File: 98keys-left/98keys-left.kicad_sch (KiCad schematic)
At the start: 115 parts, among them J1 Conn_01x04_Male, SW1 MX-NO-LED, SW10 MX-NO-LED, SW11 MX-NO-LED, SW12 MX-NO-LED, SW13 MX-NO-LED, SW14 MX-NO-LED, SW15 MX-NO-LED, SW16 MX-NO-LED, SW17 MX-NO-LED, SW18 MX-NO-LED, SW19 MX-NO-LED, SW2 MX-NO-LED, SW20 MX-NO-LED, SW21 MX-NO-LED, SW22 MX-NO-LED, SW23 MX-NO-LED, SW24 MX-NO-LED, SW25 MX-NO-LED, SW26 MX-NO-LED, SW27 MX-NO-LED, SW28 MX-NO-LED, SW29 MX-NO-LED, SW3 MX-NO-LED, SW30 MX-NO-LED, SW31 MX-NO-LED, SW32 MX-NO-LED, SW33 MX-NO-LED, SW34 MX-NO-LED, SW35 MX-NO-LED, SW36 MX-NO-LED, SW37 MX-NO-LED, SW38 MX-NO-LED, SW39 MX-NO-LED, SW4 MX-NO-LED, SW40 MX-NO-LED, SW41 MX-NO-LED, SW42 MX-NO-LED, SW43 MX-NO-LED, SW44 MX-NO-LED, SW45 MX-NO-LED, SW46 MX-NO-LED, SW47 MX-NO-LED, SW48 SW_Push, SW5 MX-NO-LED, SW6 MX-NO-LED, SW7 MX-NO-LED, SW8 MX-NO-LED, SW9 MX-NO-LED, U1 Pico

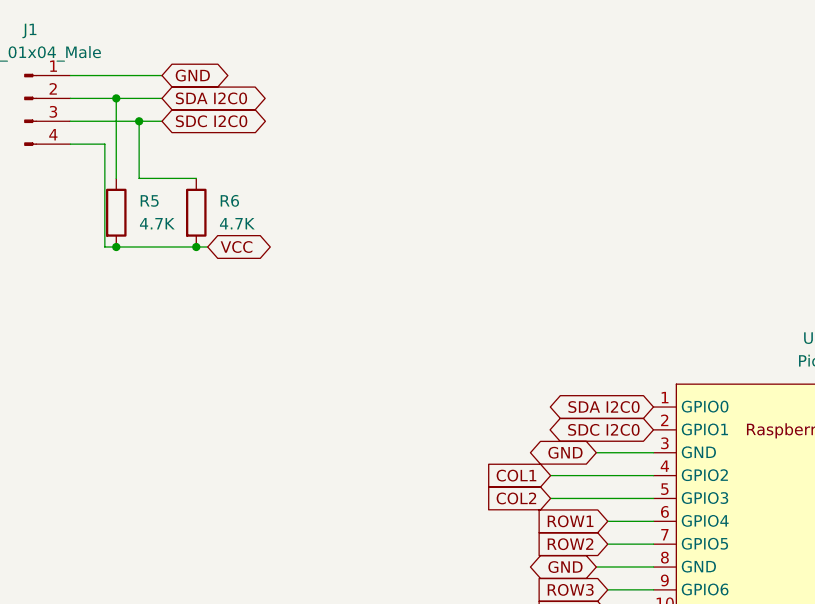
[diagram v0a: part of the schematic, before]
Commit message: Add files via upload
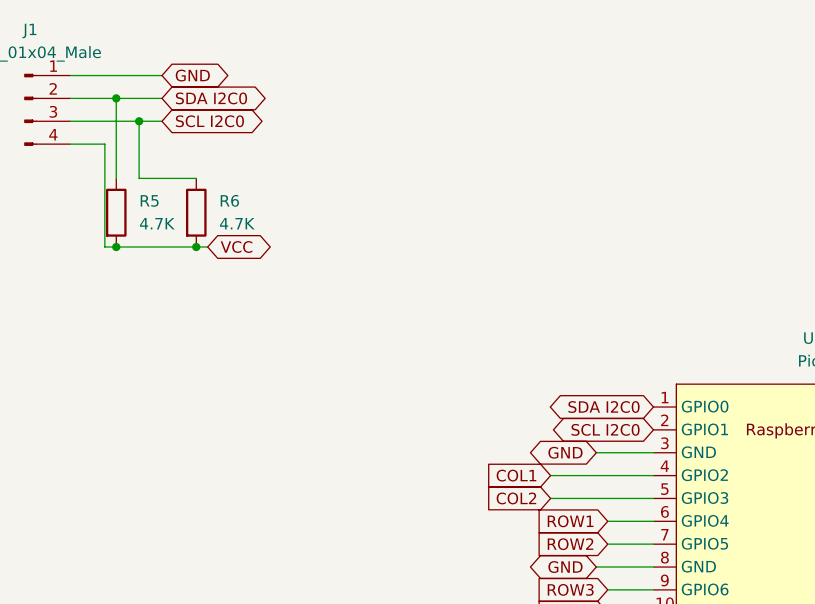
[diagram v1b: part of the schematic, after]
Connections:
- net SDC I2C0 renamed SCL I2C0
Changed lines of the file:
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@@
     )
   )
-  (global_label "SDC I2C0" (shape bidirectional) (at 495.3 86.36 180) (fields_autoplaced)
+  (global_label "SCL I2C0" (shape bidirectional) (at 495.3 86.36 180) (fields_autoplaced)
     (effects (font (size 1.27 1.27)) (justify right))
-    (property "Intersheet References" "${INTERSHEET_REFS}" (id 0) (at 483.9648 86.4394 0)
+    (property "Intersheet References" "${INTERSHEET_REFS}" (id 0) (at 484.2068 86.2806 0)
       (effects (font (size 1.27 1.27)) (justify right) hide)
     )
@@
     )
   )
-  (global_label "SDC I2C0" (shape bidirectional) (at 440.69 52.07 0) (fields_autoplaced)
+  (global_label "SCL I2C0" (shape bidirectional) (at 440.69 52.07 0) (fields_autoplaced)
     (effects (font (size 1.27 1.27)) (justify left))
-    (property "Intersheet References" "${INTERSHEET_REFS}" (id 0) (at 452.0252 51.9906 0)
+    (property "Intersheet References" "${INTERSHEET_REFS}" (id 0) (at 451.7832 51.9906 0)
       (effects (font (size 1.27 1.27)) (justify left) hide)
     )

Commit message: Add files via upload
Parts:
- J1: footprint Connector_PinHeader_2.54mm:PinHeader_1x04_P2.54mm_Vertical -> Connector_Audio:Jack_3.5mm_CUI_SJ1-43514_Horizontal
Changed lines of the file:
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@@
     (property "Reference" "J1" (id 0) (at 426.085 41.91 0))
     (property "Value" "Conn_01x04_Male" (id 1) (at 426.085 44.45 0))
-    (property "Footprint" "Connector_PinHeader_2.54mm:PinHeader_1x04_P2.54mm_Vertical" (id 2) (at 425.45 49.53 0)
+    (property "Footprint" "Connector_Audio:Jack_3.5mm_CUI_SJ1-43514_Horizontal" (id 2) (at 425.45 49.53 0)
       (effects (font (size 1.27 1.27)) hide)
     )
@@
     )
     (path "/b1a2f4f8-5ce5-4e86-9c1b-c2a387c5d74f"
-      (reference "J1") (unit 1) (value "Conn_01x04_Male") (footprint "Connector_PinHeader_2.54mm:PinHeader_1x04_P2.54mm_Vertical")
+      (reference "J1") (unit 1) (value "Conn_01x04_Male") (footprint "Connector_Audio:Jack_3.5mm_CUI_SJ1-43514_Horizontal")
     )
     (path "/00000000-0000-0000-0000-00005f7322e9"
